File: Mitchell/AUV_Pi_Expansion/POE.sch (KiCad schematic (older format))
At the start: 6 parts, among them J34 Rpi Z 1 - IN, J35 Rpi Z 2 - IN, J36 Rpi Z 3 - IN, J37 Rpi Z 1 - OUT SWITCH, J38 Rpi Z 2 - OUT SWITCH, J39 Rpi Z 3 - OUT SWITCH

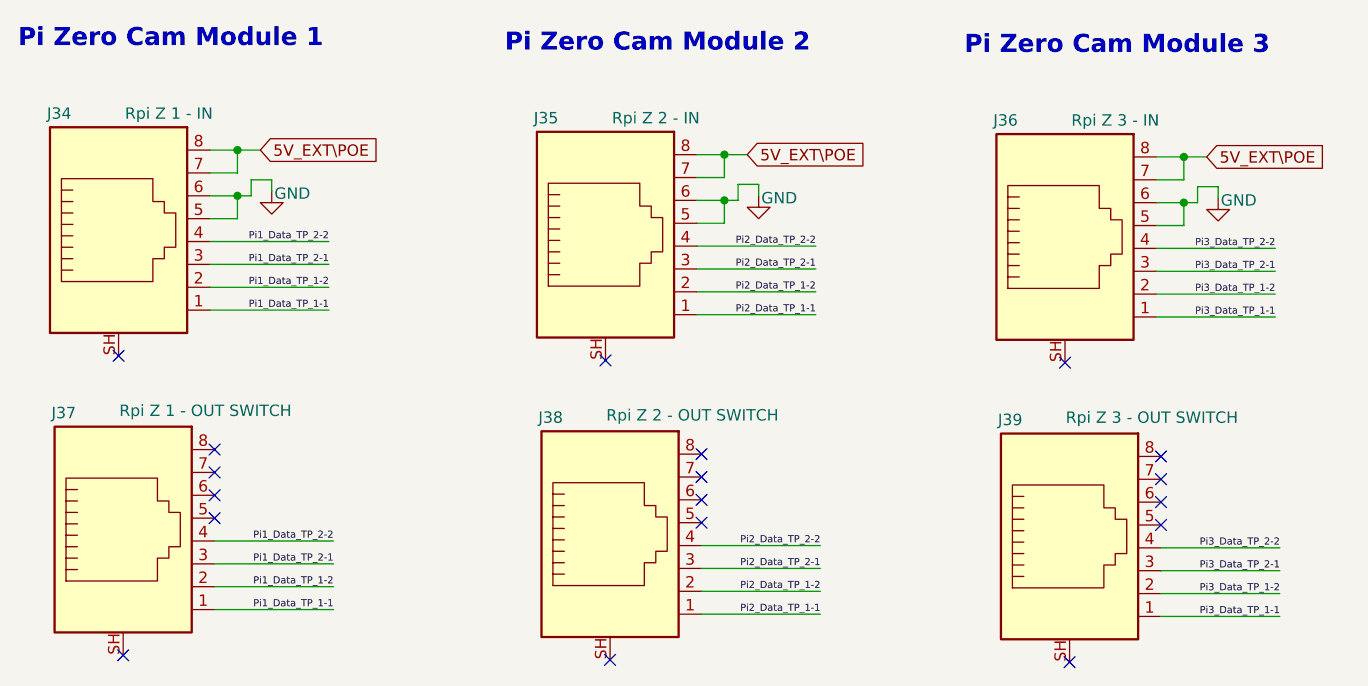
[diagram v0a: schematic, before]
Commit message: Pi4 Remake Done
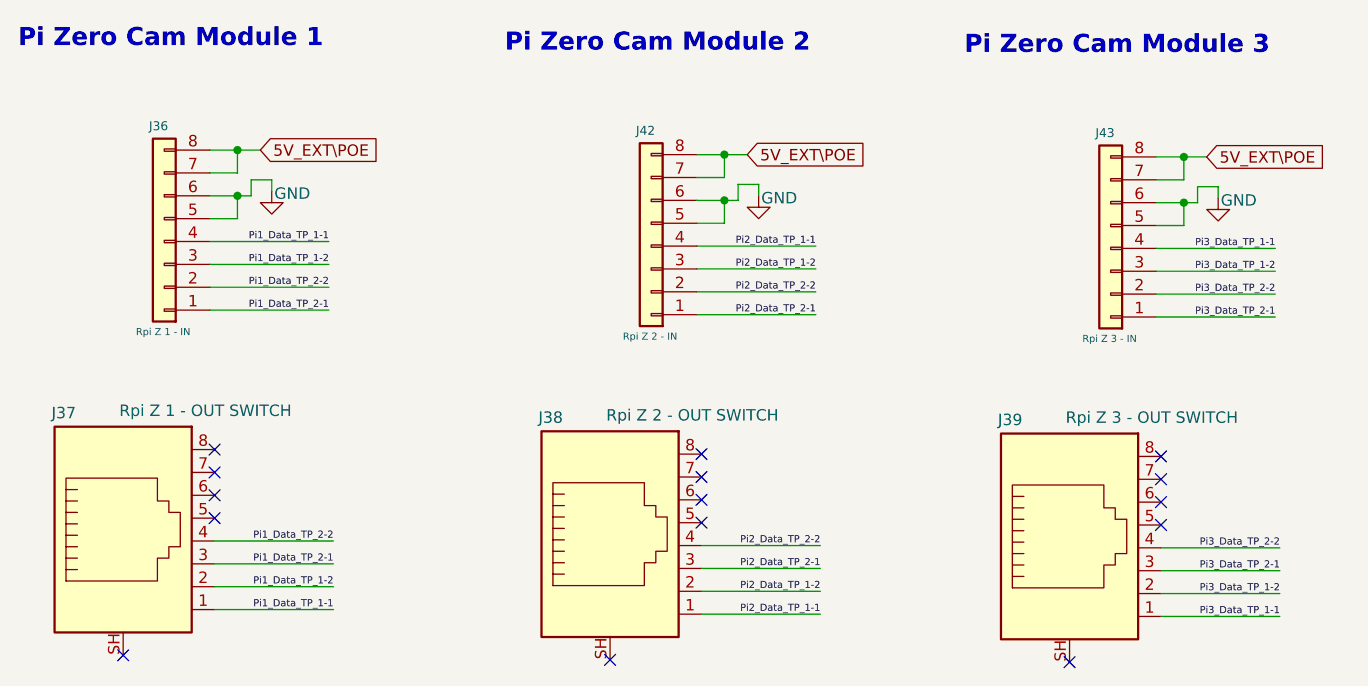
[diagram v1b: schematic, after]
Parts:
- removed J34: Rpi Z 1 - IN, µ104KiCAD_connectors:DS1128-05-S8B8P, symbol Connector:8P8C_Shielded
- removed J35: Rpi Z 2 - IN, µ104KiCAD_connectors:DS1128-05-S8B8P, symbol Connector:8P8C_Shielded
- removed J36: Rpi Z 3 - IN, µ104KiCAD_connectors:DS1128-05-S8B8P, symbol Connector:8P8C_Shielded
- added J36: Rpi Z 1 - IN, Connector_JST:JST_SH_BM08B-SRSS-TB_1x08-1MP_P1.00mm_Vertical, symbol Connector_Generic:Conn_01x08
- added J42: Rpi Z 2 - IN, Connector_JST:JST_SH_BM08B-SRSS-TB_1x08-1MP_P1.00mm_Vertical, symbol Connector_Generic:Conn_01x08
- added J43: Rpi Z 3 - IN, Connector_JST:JST_SH_BM08B-SRSS-TB_1x08-1MP_P1.00mm_Vertical, symbol Connector_Generic:Conn_01x08
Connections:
- net 5V_EXT\POE: now also J36.7 (Pin_7), J36.8 (Pin_8), J42.7 (Pin_7), J42.8 (Pin_8), J43.7 (Pin_7), J43.8 (Pin_8)
- net GND: now also J36.5 (Pin_5), J36.6 (Pin_6), J42.5 (Pin_5), J42.6 (Pin_6), J43.5 (Pin_5), J43.6 (Pin_6)
- net Pi1_Data_TP_1-1: now also J36.4 (Pin_4)
- net Pi1_Data_TP_1-2: now also J36.3 (Pin_3)
- net Pi1_Data_TP_2-1: now also J36.1 (Pin_1)
- net Pi1_Data_TP_2-2: now also J36.2 (Pin_2)
- net Pi2_Data_TP_1-1: now also J42.4 (Pin_4)
- net Pi2_Data_TP_1-2: now also J42.3 (Pin_3)
- net Pi2_Data_TP_2-1: now also J42.1 (Pin_1)
- net Pi2_Data_TP_2-2: now also J42.2 (Pin_2)
- net Pi3_Data_TP_1-1: now also J43.4 (Pin_4)
- net Pi3_Data_TP_1-2: now also J43.3 (Pin_3)
- net Pi3_Data_TP_2-1: now also J43.1 (Pin_1)
- net Pi3_Data_TP_2-2: now also J43.2 (Pin_2)
- no-connect marks 18 -> 15
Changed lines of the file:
@@
 Comment4 ""
 $EndDescr
-$Comp
-L Connector:8P8C_Shielded J34
-U 1 1 5FFF068C
-P 2470 2540
-F 0 "J34" H 2210 3100 50  0000 C CNN
-F 1 "Rpi Z 1 - IN" H 2690 3100 50  0000 C CNN
-F 2 "µ104KiCAD_connectors:DS1128-05-S8B8P" V 2470 2565 50  0001 C CNN
-F 3 "~" V 2470 2565 50  0001 C CNN
-F 4 "C86577" H 2470 2540 50  0001 C CNN "LCSC"
-F 5 "3D Model Wrong" H 2470 2540 50  0001 C CNN "Desc"
-	1    2470 2540
-	1    0    0    -1
-$EndComp
 Wire Wire Line
 	3090 2140 2990 2140
@@
 	2990 2440 2990 2340
 Wire Wire Line
-	2870 2540 3390 2540
-Text Label 3390 2540 2    31   ~ 0
+	2870 2740 3390 2740
+Text Label 3390 2740 2    31   ~ 0
 Pi1_Data_TP_2-2
 Wire Wire Line
@@
 Connection ~ 2990 2340
 Wire Wire Line
-	2870 2640 3390 2640
-Text Label 3390 2640 2    31   ~ 0
-Pi1_Data_TP_2-1
-Wire Wire Line
-	2870 2740 3390 2740
-Text Label 3390 2740 2    31   ~ 0
-Pi1_Data_TP_1-2
-Wire Wire Line
 	2870 2840 3390 2840
 Text Label 3390 2840 2    31   ~ 0
+Pi1_Data_TP_2-1
+Wire Wire Line
+	2870 2540 3390 2540
+Text Label 3390 2640 2    31   ~ 0
+Pi1_Data_TP_1-2
+Wire Wire Line
+	2870 2640 3390 2640
+Text Label 3390 2540 2    31   ~ 0
 Pi1_Data_TP_1-1
 $Comp
@@
 Text Label 3410 4150 2    31   ~ 0
 Pi1_Data_TP_1-1
-$Comp
-L Connector:8P8C_Shielded J35
-U 1 1 60018220
-P 4600 2560
-F 0 "J35" H 4340 3120 50  0000 C CNN
-F 1 "Rpi Z 2 - IN" H 4820 3120 50  0000 C CNN
-F 2 "µ104KiCAD_connectors:DS1128-05-S8B8P" V 4600 2585 50  0001 C CNN
-F 3 "~" V 4600 2585 50  0001 C CNN
-F 4 "C86577" H 4600 2560 50  0001 C CNN "LCSC"
-F 5 "3D Model Wrong" H 4600 2560 50  0001 C CNN "Desc"
-	1    4600 2560
-	1    0    0    -1
-$EndComp
 Wire Wire Line
 	5220 2160 5120 2160
@@
 	5120 2460 5120 2360
 Wire Wire Line
-	5000 2560 5520 2560
-Text Label 5520 2560 2    31   ~ 0
-Pi2_Data_TP_2-2
+	5000 2760 5520 2760
 Wire Wire Line
 	5120 2360 5180 2360
@@
 Connection ~ 5120 2360
 Wire Wire Line
-	5000 2660 5520 2660
-Text Label 5520 2660 2    31   ~ 0
-Pi2_Data_TP_2-1
-Wire Wire Line
-	5000 2760 5520 2760
-Text Label 5520 2760 2    31   ~ 0
-Pi2_Data_TP_1-2
-Wire Wire Line
 	5000 2860 5520 2860
 Text Label 5520 2860 2    31   ~ 0
+Pi2_Data_TP_2-1
+Wire Wire Line
+	5000 2560 5520 2560
+Text Label 5520 2660 2    31   ~ 0
+Pi2_Data_TP_1-2
+Wire Wire Line
+	5000 2660 5520 2660
+Text Label 5520 2560 2    31   ~ 0
 Pi2_Data_TP_1-1
 $Comp
@@
 Text Notes 4160 1720 0    79   ~ 16
 Pi Zero Cam Module 2\n
-$Comp
-L Connector:8P8C_Shielded J36
-U 1 1 6001A097
-P 6610 2570
-F 0 "J36" H 6350 3130 50  0000 C CNN
-F 1 "Rpi Z 3 - IN" H 6830 3130 50  0000 C CNN
-F 2 "µ104KiCAD_connectors:DS1128-05-S8B8P" V 6610 2595 50  0001 C CNN
-F 3 "~" V 6610 2595 50  0001 C CNN
-F 4 "C86577" H 6610 2570 50  0001 C CNN "LCSC"
-F 5 "3D Model Wrong" H 6610 2570 50  0001 C CNN "Desc"
-	1    6610 2570
-	1    0    0    -1
-$EndComp
 Wire Wire Line
 	7230 2170 7130 2170
@@
 Wire Wire Line
 	7010 2570 7530 2570
-Text Label 7530 2570 2    31   ~ 0
+Text Label 7530 2770 2    31   ~ 0
 Pi3_Data_TP_2-2
 Wire Wire Line
@@
 Wire Wire Line
 	7010 2670 7530 2670
-Text Label 7530 2670 2    31   ~ 0
+Text Label 7530 2870 2    31   ~ 0
 Pi3_Data_TP_2-1
 Wire Wire Line
 	7010 2770 7530 2770
-Text Label 7530 2770 2    31   ~ 0
-Pi3_Data_TP_1-2
 Wire Wire Line
 	7010 2870 7530 2870
-Text Label 7530 2870 2    31   ~ 0
+Text Label 7530 2570 2    31   ~ 0
 Pi3_Data_TP_1-1
 $Comp
@@
 Text GLabel 7230 2170 2    50   Input ~ 0
 5V_EXT\POE
-NoConn ~ 6610 3070
 NoConn ~ 6630 4380
 NoConn ~ 4620 4370
-NoConn ~ 4600 3060
-NoConn ~ 2470 3040
 NoConn ~ 2490 4350
+$Comp
+L Connector_Generic:Conn_01x08 J?
+U 1 1 600C8E32
+P 2670 2540
+AR Path="/5F9AFEB9/600C8E32" Ref="J?"  Part="1"
+AR Path="/600C8E32" Ref="J?"  Part="1"
+AR Path="/5F9D87DA/600C8E32" Ref="J?"  Part="1"
+AR Path="/5FCB4E5B/600C8E32" Ref="J?"  Part="1"
+AR Path="/5FFE22A4/600C8E32" Ref="J36"  Part="1"
+F 0 "J36" H 2695 2035 39  0000 C CNN
+F 1 "Rpi Z 1 - IN" H 2675 2935 31  0000 C CNN
+F 2 "Connector_JST:JST_SH_BM08B-SRSS-TB_1x08-1MP_P1.00mm_Vertical" H 2670 2540 50  0001 C CNN
+F 3 "~" H 2670 2540 50  0001 C CNN
+F 4 "C160394" H 2670 2540 50  0001 C CNN "LCSC"
+F 5 "" H 2670 2540 50  0001 C CNN "Digikey"
+F 6 "" H 2670 2540 50  0001 C CNN "Desc."
+F 7 "JST SR/SZ - SH compatible, Contact C263995, Housing C394369" H 2670 2540 50  0001 C CNN "Desc"
+	1    2670 2540
+	-1   0    0    1
+$EndComp
+$Comp
+L Connector_Generic:Conn_01x08 J?
+U 1 1 600D7A67
+P 4800 2560
+AR Path="/5F9AFEB9/600D7A67" Ref="J?"  Part="1"
+AR Path="/600D7A67" Ref="J?"  Part="1"
+AR Path="/5F9D87DA/600D7A67" Ref="J?"  Part="1"
+AR Path="/5FCB4E5B/600D7A67" Ref="J?"  Part="1"
+AR Path="/5FFE22A4/600D7A67" Ref="J42"  Part="1"
+F 0 "J42" H 4825 2055 39  0000 C CNN
+F 1 "Rpi Z 2 - IN" H 4805 2955 31  0000 C CNN
+F 2 "Connector_JST:JST_SH_BM08B-SRSS-TB_1x08-1MP_P1.00mm_Vertical" H 4800 2560 50  0001 C CNN
+F 3 "~" H 4800 2560 50  0001 C CNN
+F 4 "C160394" H 4800 2560 50  0001 C CNN "LCSC"
+F 5 "" H 4800 2560 50  0001 C CNN "Digikey"
+F 6 "" H 4800 2560 50  0001 C CNN "Desc."
+F 7 "JST SR/SZ - SH compatible, Contact C263995, Housing C394369" H 4800 2560 50  0001 C CNN "Desc"
+	1    4800 2560
+	-1   0    0    1
+$EndComp
+$Comp
+L Connector_Generic:Conn_01x08 J?
+U 1 1 600DA68F
+P 6810 2570
+AR Path="/5F9AFEB9/600DA68F" Ref="J?"  Part="1"
+AR Path="/600DA68F" Ref="J?"  Part="1"
+AR Path="/5F9D87DA/600DA68F" Ref="J?"  Part="1"
+AR Path="/5FCB4E5B/600DA68F" Ref="J?"  Part="1"
+AR Path="/5FFE22A4/600DA68F" Ref="J43"  Part="1"
+F 0 "J43" H 6835 2065 39  0000 C CNN
+F 1 "Rpi Z 3 - IN" H 6815 2965 31  0000 C CNN
+F 2 "Connector_JST:JST_SH_BM08B-SRSS-TB_1x08-1MP_P1.00mm_Vertical" H 6810 2570 50  0001 C CNN
+F 3 "~" H 6810 2570 50  0001 C CNN
+F 4 "C160394" H 6810 2570 50  0001 C CNN "LCSC"
+F 5 "" H 6810 2570 50  0001 C CNN "Digikey"
+F 6 "" H 6810 2570 50  0001 C CNN "Desc."
+F 7 "JST SR/SZ - SH compatible, Contact C263995, Housing C394369" H 6810 2570 50  0001 C CNN "Desc"
+	1    6810 2570
+	-1   0    0    1
+$EndComp
+Text Label 7530 2670 2    31   ~ 0
+Pi3_Data_TP_1-2
+Text Label 5520 2760 2    31   ~ 0
+Pi2_Data_TP_2-2
 $EndSCHEMATC
